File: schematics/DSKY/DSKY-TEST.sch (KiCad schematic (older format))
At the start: 7 parts, among them J203 Conn_02x08, J204 Conn_02x10, J300 RPI_Connector, U100 74HC245, U101 74HC245, U102 74HC245, U103 74HC245

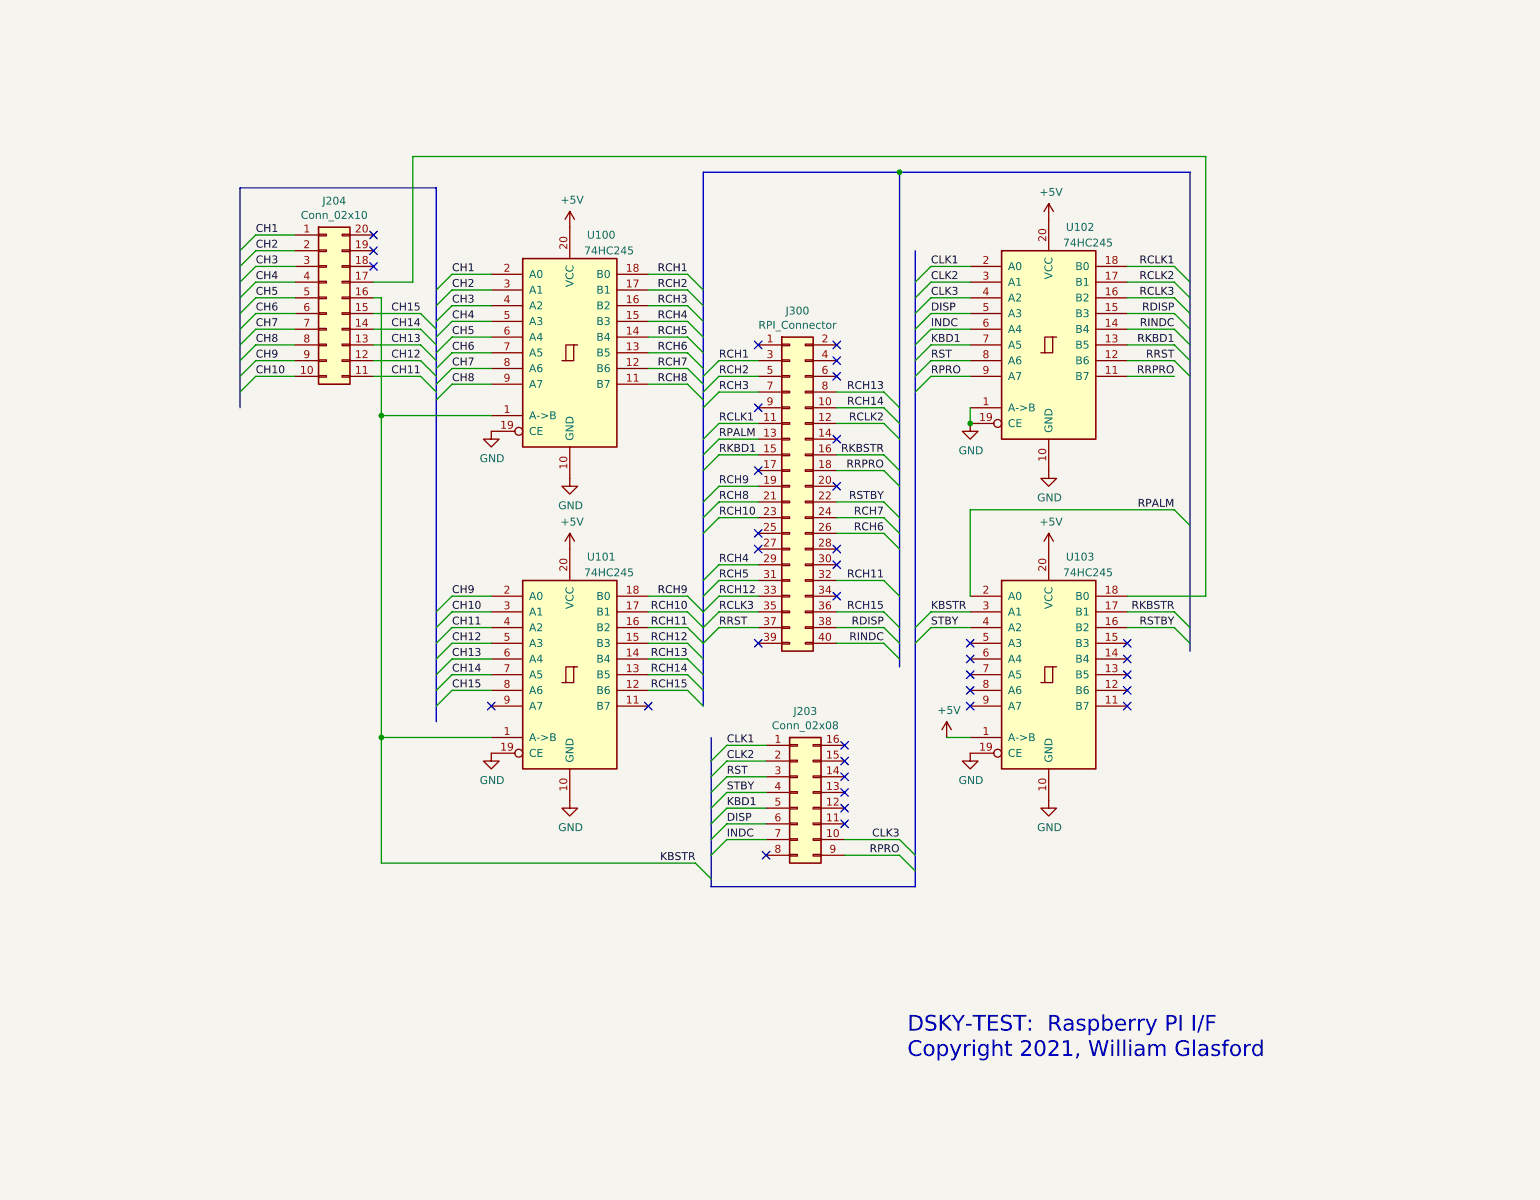
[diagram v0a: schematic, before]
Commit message: DSKY Redesign
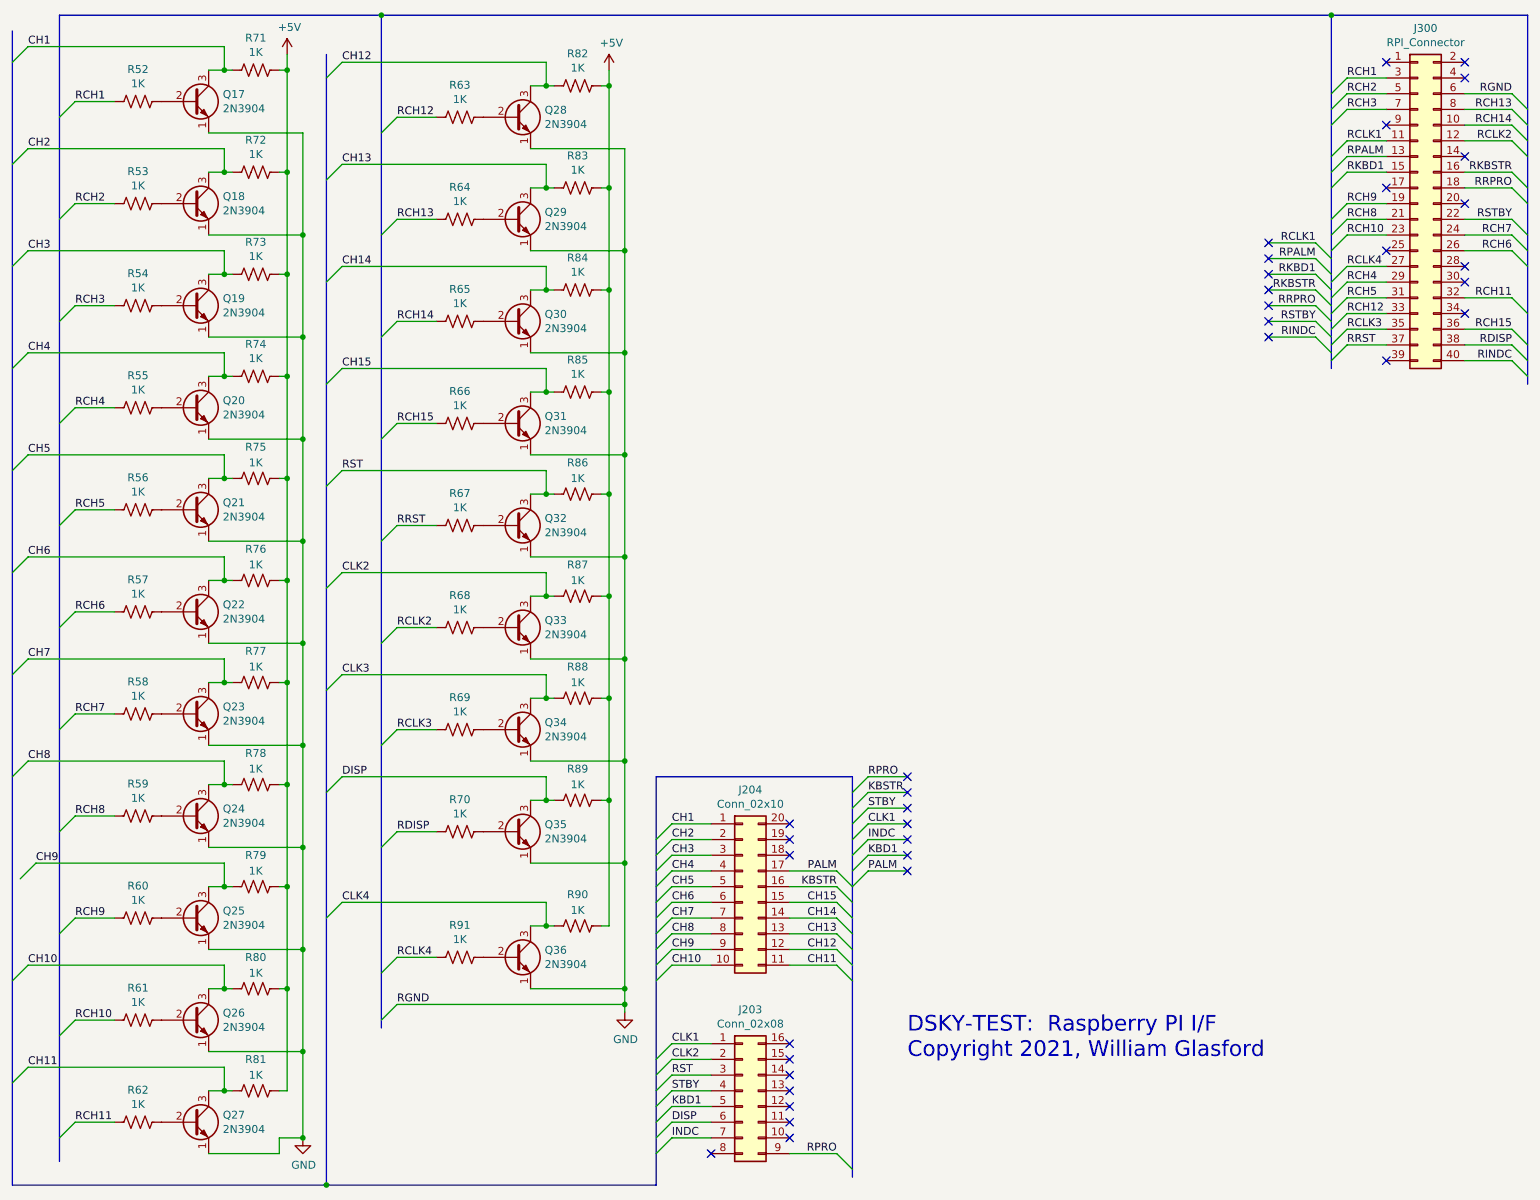
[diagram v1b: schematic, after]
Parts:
- removed U100, U101, U102, U103: 74HC245, symbol 74xx:74HC245
- added Q17, Q18, Q19, Q20, Q21, Q22, Q23, Q24, Q25, Q26, Q27, Q28, Q29, Q30, Q31, Q32, Q33, Q34, Q35, Q36: 2N3904, Package_TO_SOT_THT:TO-92_Inline, symbol Transistor_BJT:2N3904
- added R52, R53, R54, R55, R56, R57, R58, R59, R60, R61, R62, R63, R64, R65, R66, R67, R68, R69, R70, R71, R72, R73, R74, R75, R76, R77, R78, R79, R80, R81, R82, R83, R84, R85, R86, R87, R88, R89, R90, R91: 1K, symbol Device:R_US
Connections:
- net +5V: now also R71.1, R72.1, R73.1, R74.1, R75.1, R76.1, R77.1, R78.1, R79.1, R80.1, R81.1, R82.1, R83.1, R84.1, R85.1, R86.1, R87.1, R88.1, R89.1, R90.1
- net CH1: now also Q17.3 (C), R71.2
- net CH10: now also Q26.3 (C), R80.2
- net CH11: now also Q27.3 (C), R81.2
- net CH12: now also Q28.3 (C), R82.2
- net CH13: now also Q29.3 (C), R83.2
- net CH14: now also Q30.3 (C), R84.2
- net CH15: now also Q31.3 (C), R85.2
- net CH2: now also Q18.3 (C), R72.2
- net CH3: now also Q19.3 (C), R73.2
- net CH4: now also Q20.3 (C), R74.2
- net CH5: now also Q21.3 (C), R75.2
- net CH6: now also Q22.3 (C), R76.2
- net CH7: now also Q23.3 (C), R77.2
- net CH8: now also Q24.3 (C), R78.2
- net CH9: now also Q25.3 (C), R79.2
- net CLK2: now also Q33.3 (C), R87.2
- net CLK3: now also Q34.3 (C), R88.2; no longer J203.10 (Pin_10)
- net DISP: now also Q35.3 (C), R89.2
- net GND: now also J300.6 (Pin_6), Q17.1 (E), Q18.1 (E), Q19.1 (E), Q20.1 (E), Q21.1 (E), Q22.1 (E), Q23.1 (E), Q24.1 (E), Q25.1 (E), Q26.1 (E), Q27.1 (E), Q28.1 (E), Q29.1 (E), Q30.1 (E), Q31.1 (E), Q32.1 (E), Q33.1 (E), Q34.1 (E), Q35.1 (E), Q36.1 (E)
- net RCH1: now also R52.2
- net RCH10: now also R61.2
- net RCH11: now also R62.2
- net RCH12: now also R63.2
- net RCH13: now also R64.2
- net RCH14: now also R65.2
- net RCH15: now also R66.2
- net RCH2: now also R53.2
- net RCH3: now also R54.2
- net RCH4: now also R55.2
- net RCH5: now also R56.2
- net RCH6: now also R57.2
- net RCH7: now also R58.2
- net RCH8: now also R59.2
- net RCH9: now also R60.2
- net RCLK2: now also R68.2
- net RCLK3: now also R69.2
- net RDISP: now also R70.2
- net RRST: now also R67.2
- net RST: now also Q32.3 (C), R86.2
- net PALM: now reaches J204.17 (Pin_17)
- net RCLK4: now reaches J300.27 (Pin_27)
- net RCLK4: now also R91.2
- new net: Q20.2 (B), R55.1
- new net: Q21.2 (B), R56.1
- new net: Q19.2 (B), R54.1
- new net: Q18.2 (B), R53.1
- new net: Q17.2 (B), R52.1
- new net: Q22.2 (B), R57.1
- new net: Q23.2 (B), R58.1
- new net: Q24.2 (B), R59.1
- new net: Q25.2 (B), R60.1
- new net: Q26.2 (B), R61.1
- new net: Q27.2 (B), R62.1
- new net: Q31.2 (B), R66.1
- new net: Q32.2 (B), R67.1
- new net: Q30.2 (B), R65.1
- new net: Q29.2 (B), R64.1
- new net: Q28.2 (B), R63.1
- new net: Q33.2 (B), R68.1
- new net: Q34.2 (B), R69.1
- new net: Q35.2 (B), R70.1
- new net: Q36.2 (B), R91.1
- new net CLK4: Q36.3 (C), R90.2
- no-connect marks 36 -> 37
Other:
- moved on the sheet: J203, J204, J300
